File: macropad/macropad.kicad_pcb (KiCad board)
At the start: 2 copper layers, 77.5 x 61 mm, 45 parts, among them IC1 W25Q16JVUXIQ_TR, J1 Conn_01x03_Female, J2 USB_C_Receptacle, SW1 BOOT, SW2 RESET, U1 RP2040, U10 DRV5056A2, U11 DRV5056A2, U12 OLED_256x64_I2C, U2 DRV5056A2, U3 DRV5056A2, U4 DRV5056A2, U5 DRV5056A2, U6 CD74HC4067SM96E4, U7 DRV5056A2, U8 DRV5056A2, U9 NCP1117-3.3_SOT223, Y1 ECS-120-8-30-JGN-TR

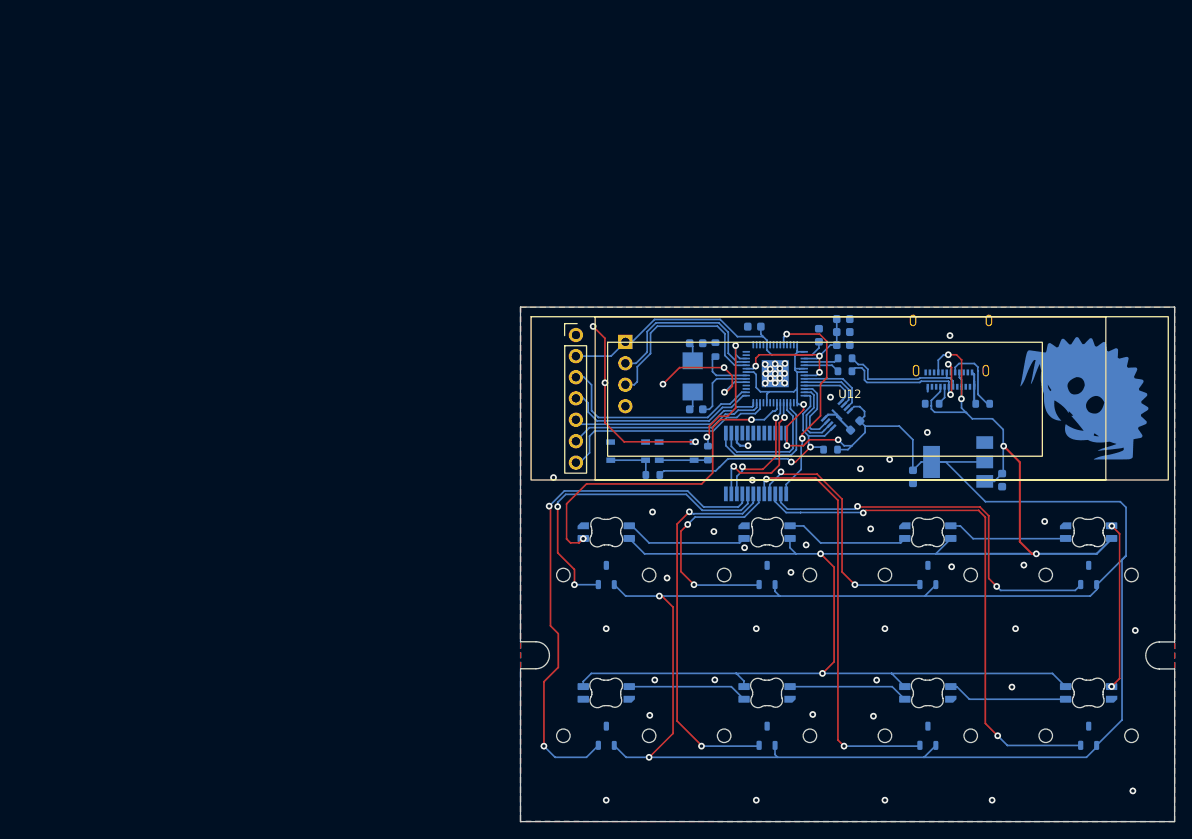
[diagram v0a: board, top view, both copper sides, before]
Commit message: whatever the fuck i all did
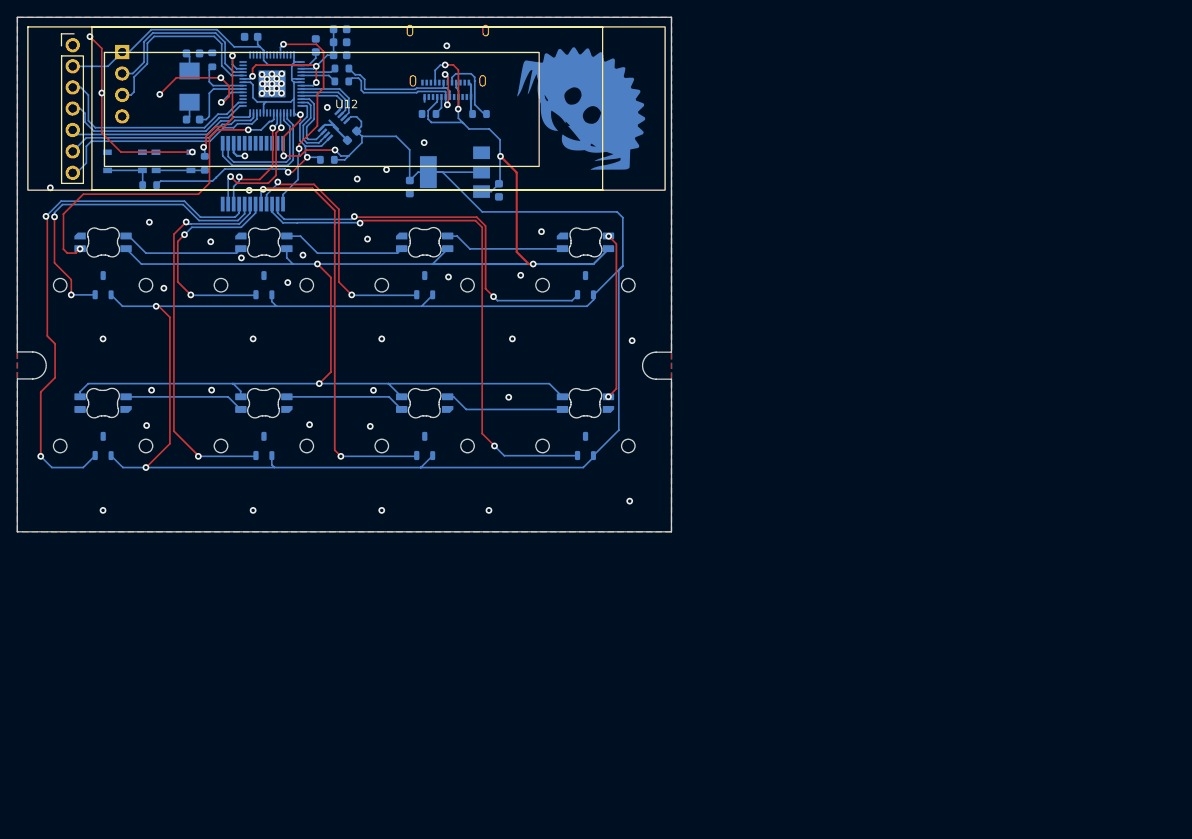
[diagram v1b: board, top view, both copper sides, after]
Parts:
- moved C2 68.8 mm to (82.9, 42.4)
- moved C3 68.8 mm to (82.9, 50.2)
- moved C4 68.8 mm to (97.4, 41.4)
- moved C6 68.8 mm to (119.1, 58.6)
- moved C8 68.8 mm to (89.8, 40.4)
- moved IC1 68.8 mm to (99.6, 50.9)
- moved J1 68.8 mm to (74.5, 42.2)
- moved J2 68.8 mm to (113.1, 42.5)
- moved LED3 68.8 mm to (91.3, 69.9)
- moved LED4 68.8 mm to (91.3, 88.9)
- moved LED7 68.8 mm to (129.4, 69.9)
- moved LED8 68.8 mm to (129.4, 88.9)
- moved R3 68.8 mm to (85.2, 43.1)
- moved R5 68.8 mm to (100.5, 45.7)
- moved R6 68.8 mm to (116.8, 49.6)
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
